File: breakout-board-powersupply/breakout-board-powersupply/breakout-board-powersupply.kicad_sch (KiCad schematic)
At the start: 15 parts, among them J1 Screw_Terminal_01x02, J2 Conn_01x05_Female, T1 Transformer_1P_1S, U1 L7805

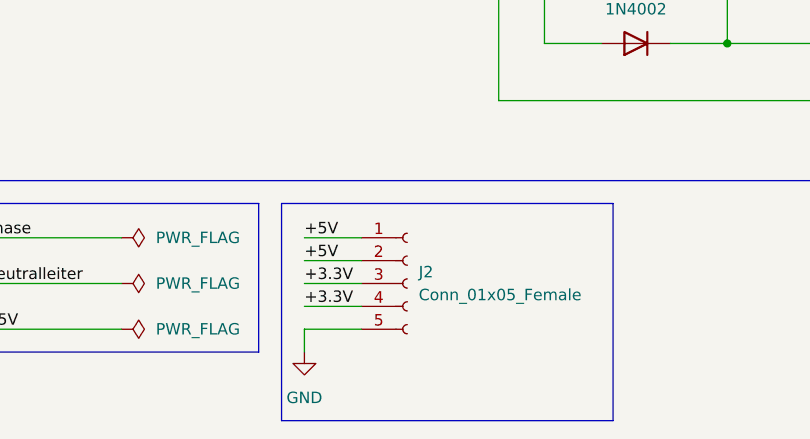
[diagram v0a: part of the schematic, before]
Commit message: Revert "..."
This reverts commit 6093de15b6a411821706cd1d809fe7ad2ca1dc62.
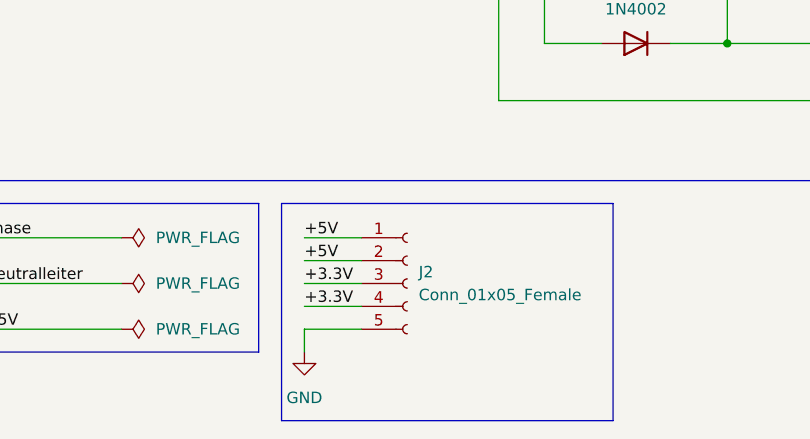
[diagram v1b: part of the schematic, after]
